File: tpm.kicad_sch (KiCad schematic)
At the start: 1 part, among them J8 TFM-107-01-X-D-RE1-WT

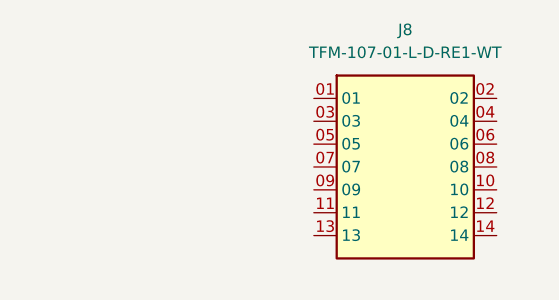
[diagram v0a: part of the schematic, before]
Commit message: Annotate schematic
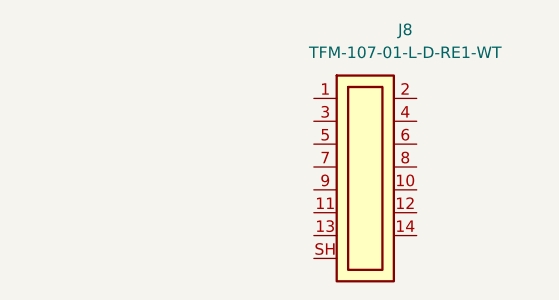
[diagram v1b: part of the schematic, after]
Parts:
- J8: footprint antmicro-footprints:Socket_Samtec_TFM_2x7_TFM-107-01-X-D-RE1-WT -> antmicro-footprints:Conn_Socket_Samtec_TFM_2x7_TFM-107-01-X-D-RE1-WT
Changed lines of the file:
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@@
 			)
 		)
-		(property "Footprint" "antmicro-footprints:Socket_Samtec_TFM_2x7_TFM-107-01-X-D-RE1-WT"
+		(property "Footprint" "antmicro-footprints:Conn_Socket_Samtec_TFM_2x7_TFM-107-01-X-D-RE1-WT"
 			(at 210.82 97.79 0)
 			(effects
@@
 			)
 		)
-		(pin "06"
+		(pin "2"
 		)
 		(pin "12"
@@
 		(pin "11"
 		)
-		(pin "09"
+		(pin "1"
 		)
-		(pin "07"
+		(pin "6"
 		)
-		(pin "05"
+		(pin "9"
 		)
-		(pin "03"
+		(pin "8"
 		)
-		(pin "01"
+		(pin "3"
 		)
-		(pin "02"
+		(pin "4"
 		)
-		(pin "04"
+		(pin "5"
 		)
 		(pin "14"
@@
 		(pin "10"
 		)
-		(pin "08"
+		(pin "7"
+		)
+		(pin "SH"
 		)
 		(instances
